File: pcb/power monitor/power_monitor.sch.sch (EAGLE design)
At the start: 14 parts, among them IC1 MAX4105ESA, IC2 MAX4105ESA, IC3 MAX4105ESA

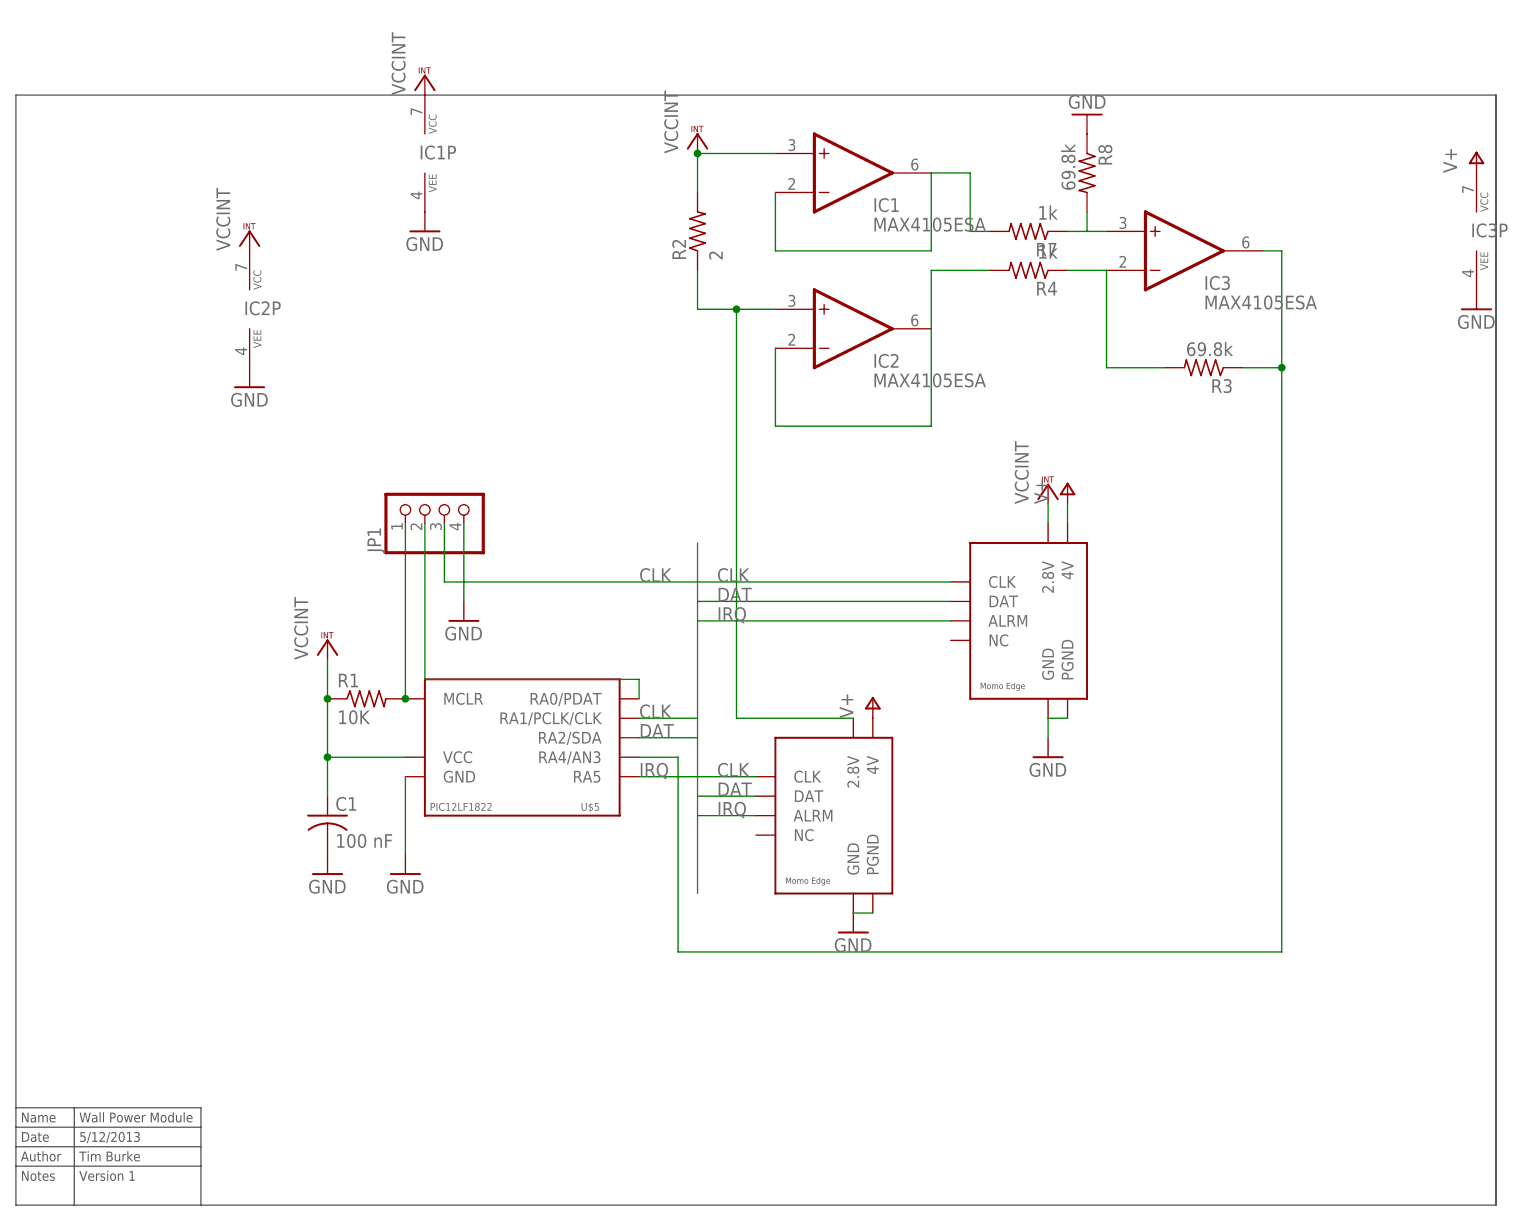
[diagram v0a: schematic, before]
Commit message: Signed-off-by: timcronin <tmpcronin@gmail.com>
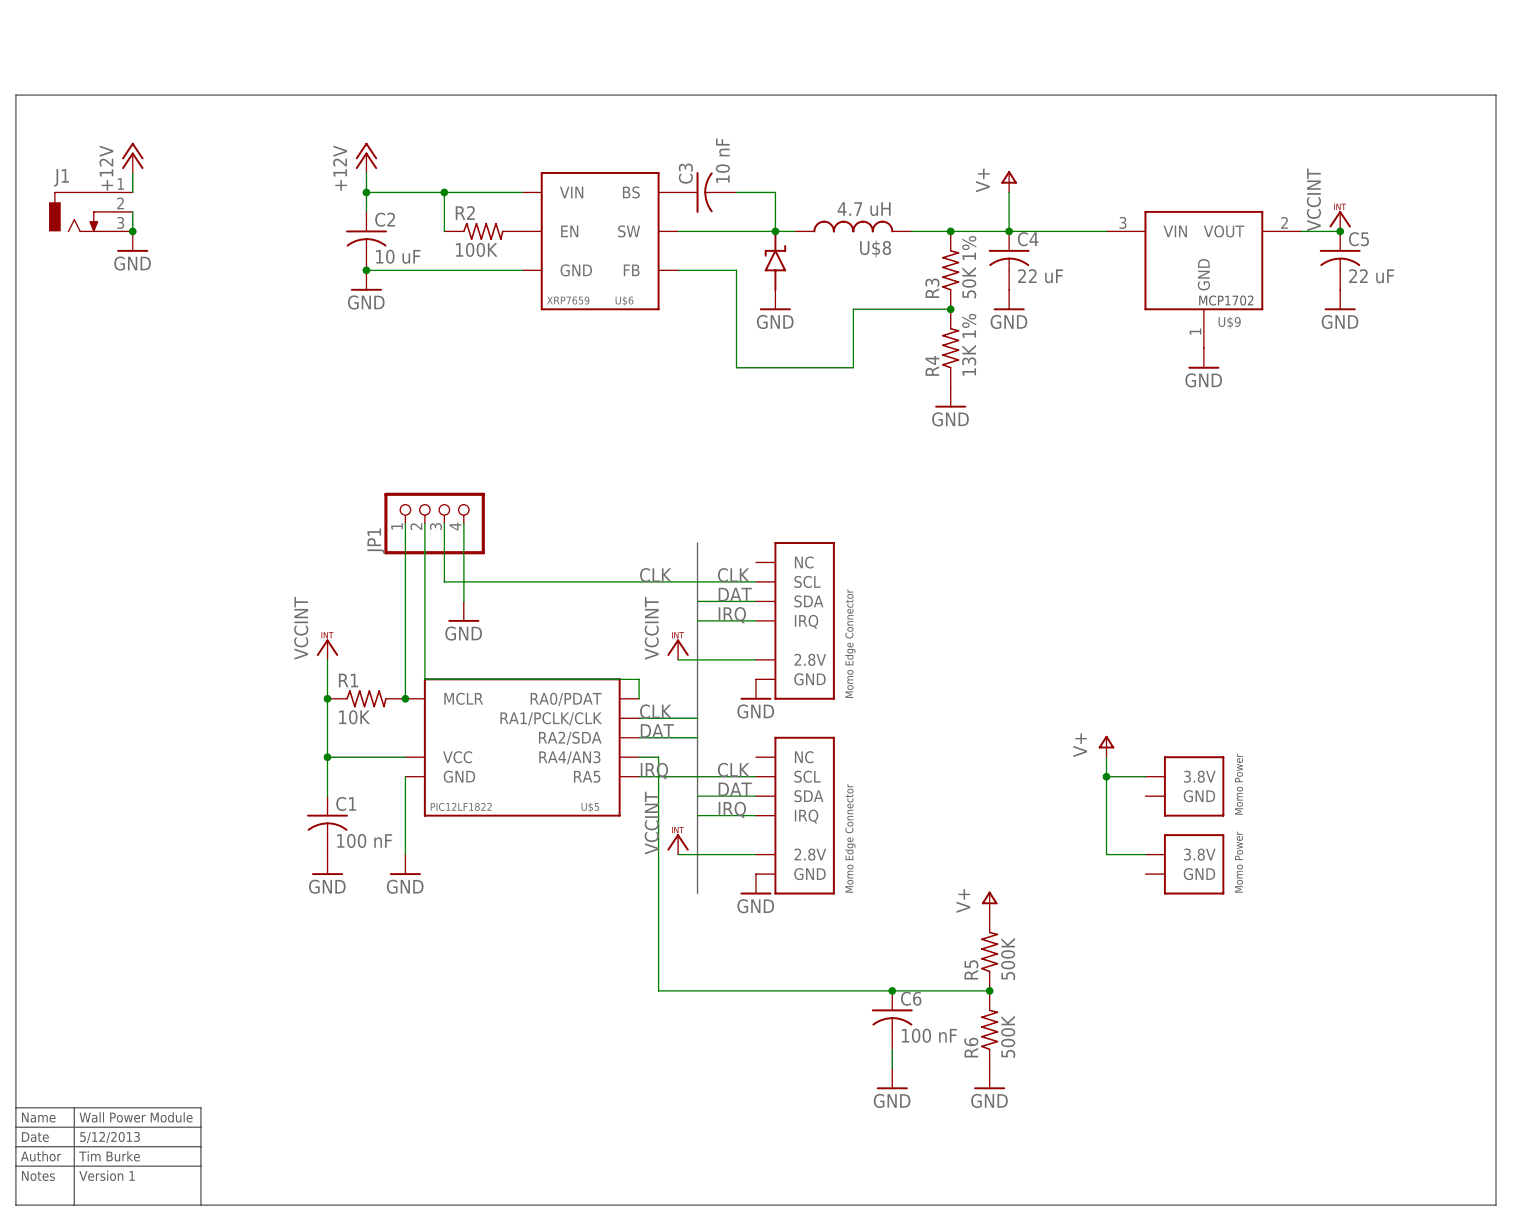
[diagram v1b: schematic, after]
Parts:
- removed IC1, IC2, IC3: MAX4105ESA, maxim:MAX4105ESA
- removed R7: 1k, rcl:R-US_R0603
- removed R8: 69.8k, rcl:R-US_R0603
- added C2: 10 uF, rcl:C-USC0805
- added C3: 10 nF, rcl:C-USC0402
- added C4: 22 uF, rcl:C-USC1206
- added C5: 22 uF, rcl:C-USC0402
- added C6: 100 nF, rcl:C-USC0402
- added J1: (no value), con-jack:DCJ0303
- added R5, R6: 500K, rcl:R-US_R0603
- added U$1: MOMO-EDGE-SMALL-M, components:MOMO-EDGE-SMALL-M
- added U$2: MOMO-EDGE-SMALL-F, components:MOMO-EDGE-SMALL-F
- added U$3: MOMO-EDGE-POWER-M, components:MOMO-EDGE-POWER-M
- added U$4: MOMO-EDGE-POWER-F, components:MOMO-EDGE-POWER-F
- added U$8: 4.7 uH, components:NR6028-INDUCTOR
- added U$9: MCP1702, components:MCP1702
- R2: value 2 -> 100K
- R3: value 69.8k -> 50K 1%
- R4: value 1k -> 13K 1%
- U$6: value MOMO-EDGE-8F -> XRP7659; device components:MOMO-EDGE-8F -> components:XRP7659
- U$7: value MOMO-EDGE-8M -> DIODE_SS2P3; device components:MOMO-EDGE-8M -> components:DIODE_SS2P3
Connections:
- removed net N$11: IC2G$1.+IN, R2.1, U$7.2.8V
- removed net N$7: IC3G$1.-IN, R3.2, R4.1
- removed net N$9: IC3G$1.+IN, R7.1, R8.2
- new net +12V: C2.1, J1.1, R2.1, U$6.VIN
- new net N$5: C6.1, R5.1, R6.2, U$5.RA4/AN3
- new net N$6: R3.1, R4.2, U$6.FB
- net CLK: now also U$1.SCL, U$2.SCL; no longer U$6.CLK, U$7.CLK
- net DAT: now also U$1.SDA, U$2.SDA; no longer U$6.DAT, U$7.DAT
- net GND: now also C2.2, C4.2, C5.2, C6.2, J1.2, J1.3, R4.1, R6.1, U$1.GND, U$2.GND, U$7.AN, U$9.GND; no longer IC1P.VEE, IC2P.VEE, IC3P.VEE, R8.1, U$6.PGND, U$7.GND, U$7.PGND
- net IRQ: now also U$1.IRQ, U$2.IRQ; no longer U$6.ALRM, U$7.ALRM
- net N$2: now also C3.2, U$6.SW, U$7.CATH, U$8.1; no longer IC3G$1.OUT, R3.1, U$5.RA4/AN3
- net N$3: now also R2.2, U$6.EN; no longer IC2G$1.-IN, IC2G$1.OUT, R4.2
- net N$4: now also C3.1, U$6.BS; no longer IC1G$1.-IN, IC1G$1.OUT, R7.2
- net V+: now also C4.1, R3.2, R5.2, U$3.3.8V, U$4.3.8V, U$8.2, U$9.VIN; no longer IC3P.VCC, U$6.4V, U$7.4V
- net VCCINT: now also C5.1, U$1.2.8V, U$2.2.8V, U$9.VOUT; no longer IC1G$1.+IN, IC1P.VCC, IC2P.VCC, R2.2, U$6.2.8V
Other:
- moved on the sheet: R2, R3, R4
